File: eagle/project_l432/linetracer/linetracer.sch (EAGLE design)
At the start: 2 parts

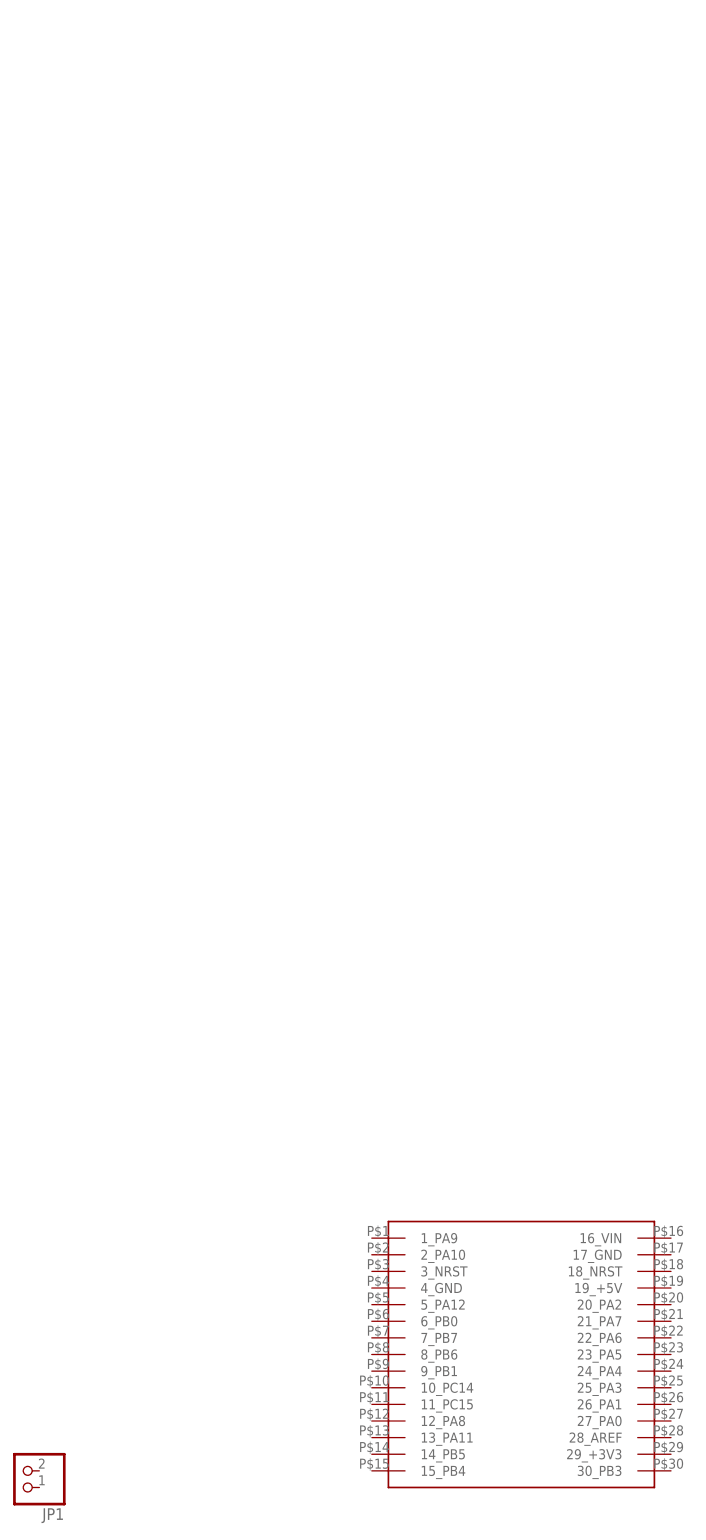
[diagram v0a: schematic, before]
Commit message: power
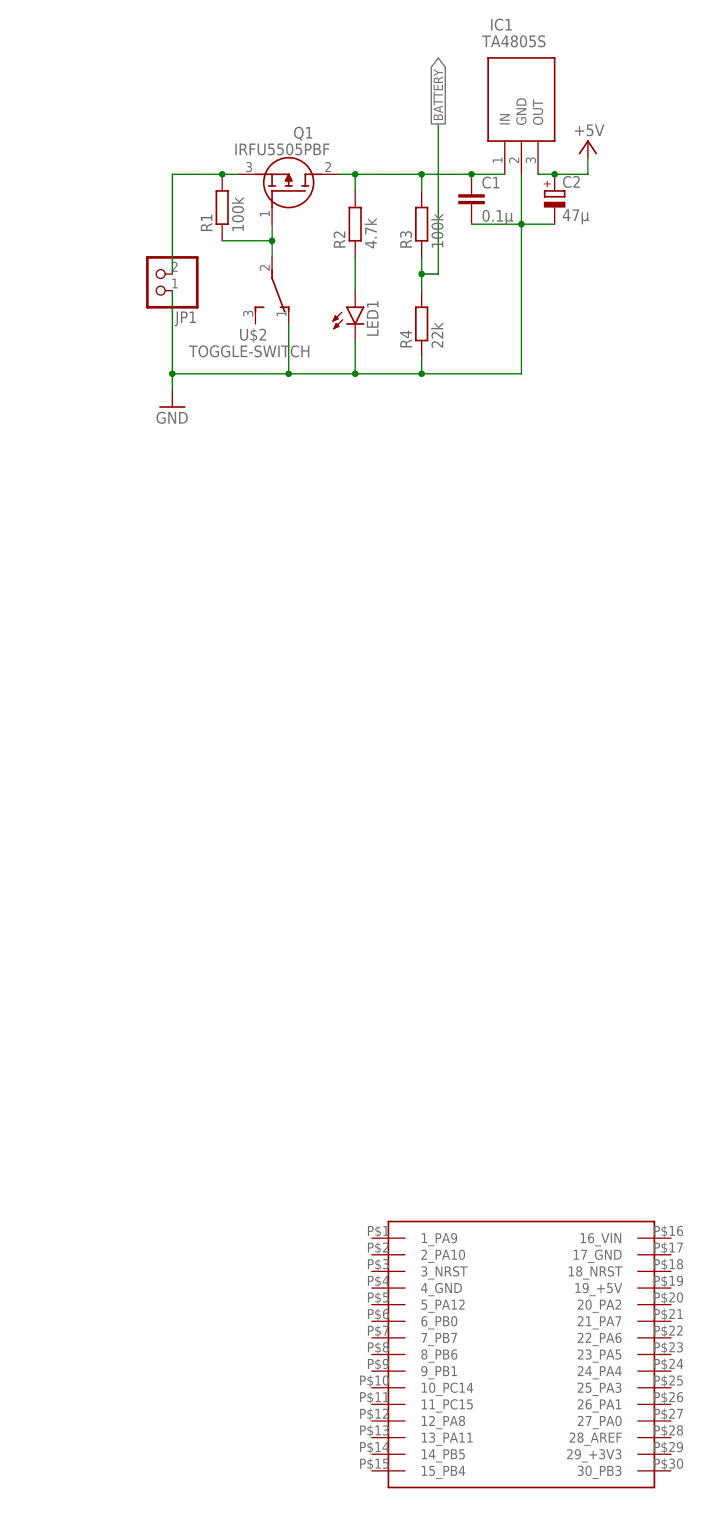
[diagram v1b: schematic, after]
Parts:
- added C1: 0.1μ, rcl:C-EU025-024X044
- added C2: 47μ, rcl:CPOL-EUE5-10.5
- added IC1: TA4805S, TA4805S:TA4805S
- added LED1: (no value), led:LED3MM
- added Q1: IRFU5505PBF, IRFU5505PBF:IRFU5505PBF
- added R1, R3: 100k, rcl:R-EU_0204/2V
- added R2: 4.7k, rcl:R-EU_0204/2V
- added R4: 22k, rcl:R-EU_0204/2V
- added U$2: TOGGLE-SWITCH, toggle-switch:TOGGLE-SWITCH
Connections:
- new net +5V: C2.+, IC1.OUT
- new net BATTERY: R3.1, R4.2
- new net GND: C1.2, C2.-, IC1.GND, JP1.1, LED1.C, R4.1, U$2.1
- new net N$1: JP1.2, Q1.S, R1.2
- new net N$2: Q1.G, R1.1, U$2.2
- new net N$4: C1.1, IC1.IN, Q1.D, R2.2, R3.2
- new net N$5: LED1.A, R2.1
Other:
- moved on the sheet: JP1
